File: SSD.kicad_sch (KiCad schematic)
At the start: 10 parts, among them J7 1935174, K1 EE2-12SNUH, Q1 BSP296NH6327XTSA1

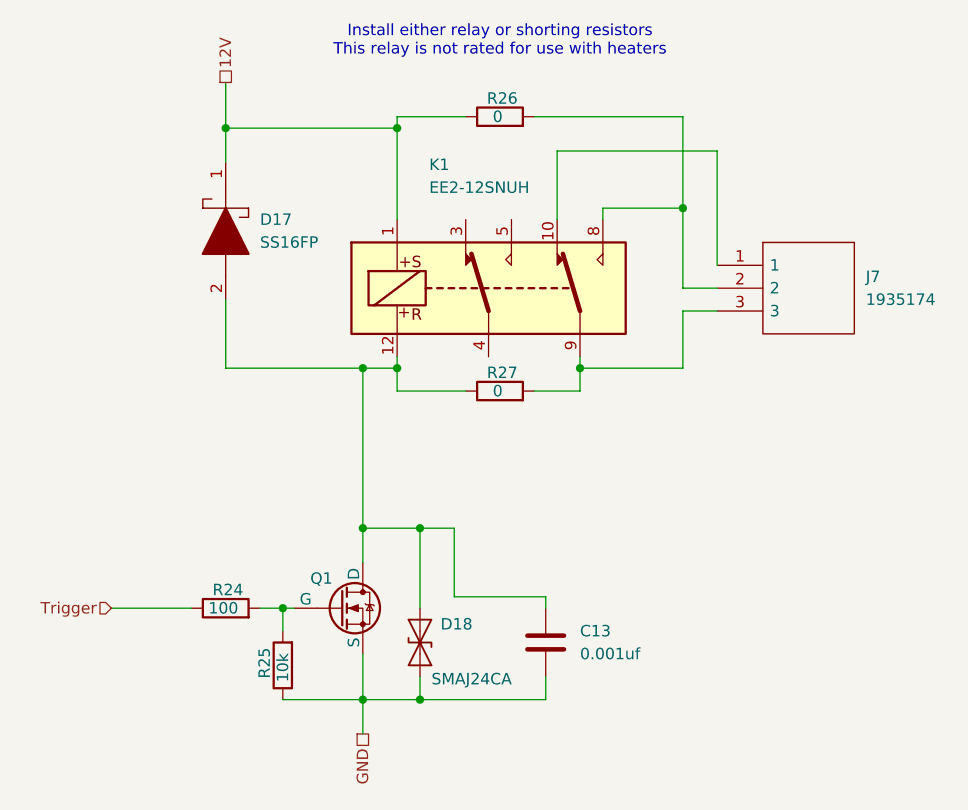
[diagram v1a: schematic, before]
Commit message: sch progress
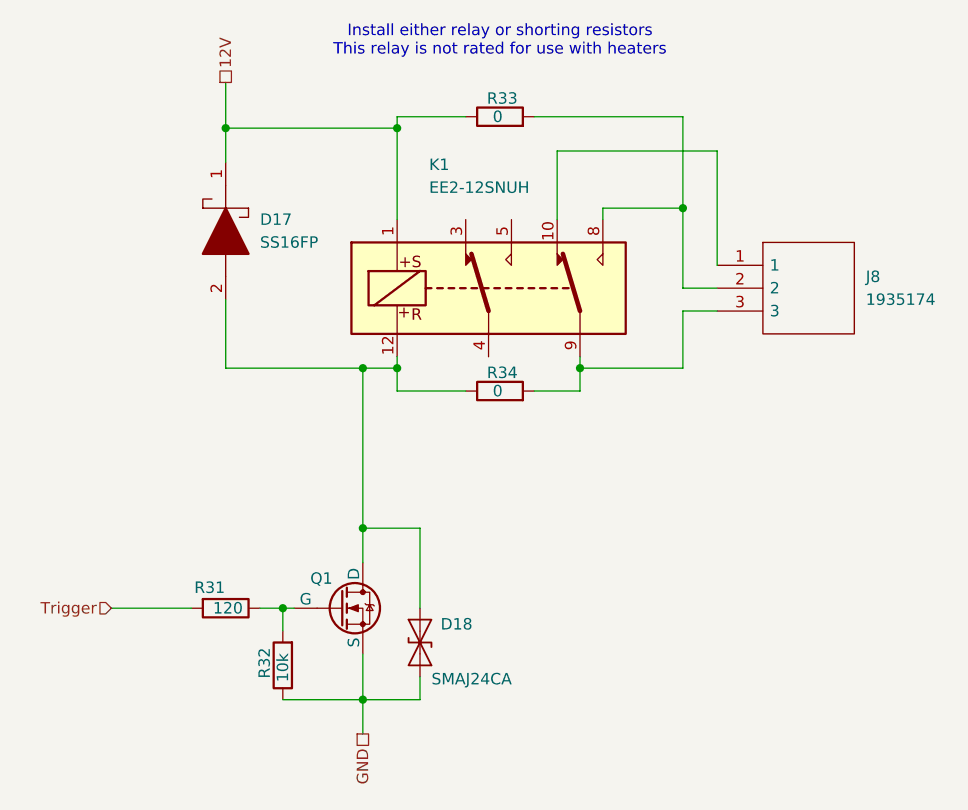
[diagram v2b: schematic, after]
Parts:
- removed C13: 0.001uf, Capacitor_SMD:C_0402_1005Metric, symbol Device:C
- removed R24: 100, Resistor_SMD:R_0402_1005Metric, symbol Device:R
- added R31: 120, Resistor_SMD:R_0402_1005Metric, symbol Device:R
- renumbered J7 to J8, R25 to R32, R26 to R33, R27 to R34
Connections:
- net Trigger: now also R31.2
- net at Q1.2 (G), R32.2: now also R31.1
